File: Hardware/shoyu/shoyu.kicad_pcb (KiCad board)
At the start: 2 copper layers, 58 parts, among them J1 5/9V Connector, J2 24V Connector, J3 SHORI OUT, J4 GAMEN_OUT, J5 MAE OUT, J6 AUDIO IN, U1 TPA3255DDVR, U2 TSR 1-24120

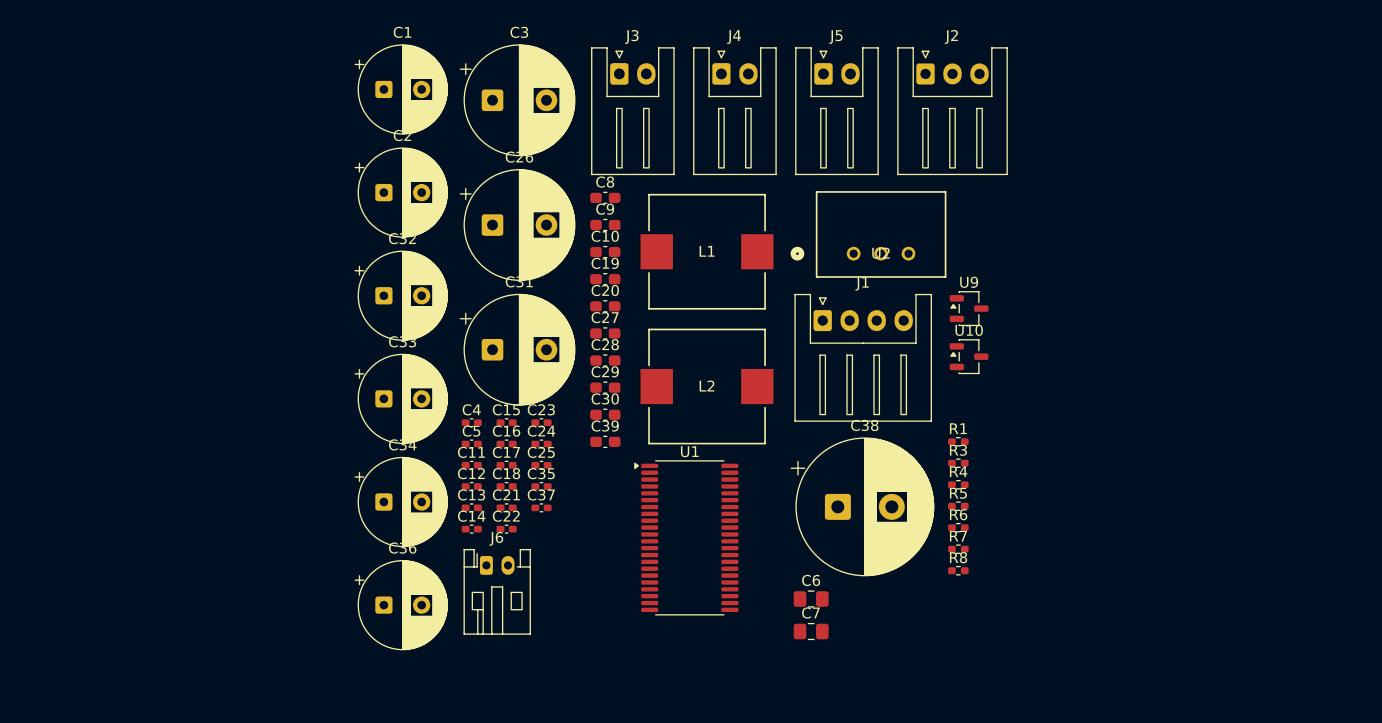
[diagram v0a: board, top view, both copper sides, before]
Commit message: Shoyu: Layout complete
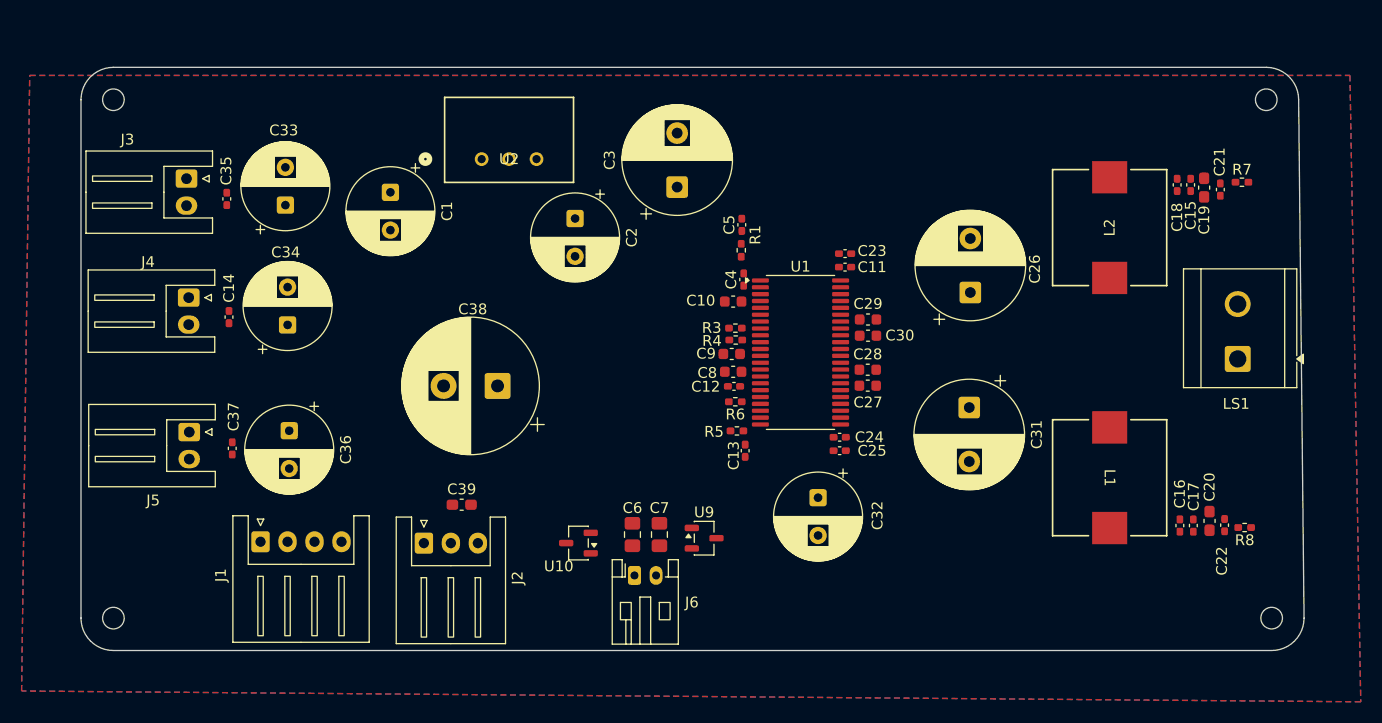
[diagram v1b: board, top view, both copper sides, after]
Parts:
- added H1: MountingHole, MountingHole:MountingHole_2mm, F.Cu at (95.8, 78.0)
- added H2: MountingHole, MountingHole:MountingHole_2mm, F.Cu at (95.8, 126.0)
- added H3: MountingHole, MountingHole:MountingHole_2mm, F.Cu at (202.5, 78.0)
- added H4: MountingHole, MountingHole:MountingHole_2mm, F.Cu at (203.0, 126.0)
- added LS1: Speaker, TerminalBlock_CUI:TerminalBlock_CUI_TB007-508-02_1x02_P5.08mm_Horizontal, F.Cu at (199.9, 102.0)
- C10, C8, C9: footprint Capacitor_SMD:C_0603_1608Metric_Pad1.08x0.95mm_HandSolder -> Capacitor_SMD:C_0603_1608Metric
- C27, C28, C29, C30: value 1uF -> 2.2uF; footprint Capacitor_SMD:C_0603_1608Metric_Pad1.08x0.95mm_HandSolder -> Capacitor_SMD:C_0603_1608Metric
- U2: footprint My Footprints:TSR1-SINGLE_TRP -> My Feet pics:TSR1-SINGLE_TRP
- moved C21 72.4 mm to (198.2, 86.3), turned to -90 degrees
- moved C18 68.1 mm to (194.2, 85.9), turned to 90 degrees
- moved J5 67.4 mm to (102.8, 108.8), turned to -90 degrees
- moved C15 67.1 mm to (195.5, 85.9), turned to 90 degrees
- moved C22 66.5 mm to (198.6, 117.4), turned to -90 degrees
- moved C17 63.8 mm to (195.8, 117.4), turned to 90 degrees
- moved J2 63.6 mm to (124.5, 119.1)
- moved C16 62.8 mm to (194.5, 117.4), turned to 90 degrees
- moved C20 59.4 mm to (197.2, 117.0), turned to 90 degrees
- moved C19 56.1 mm to (196.8, 86.1), turned to 90 degrees
- moved J1 55.9 mm to (109.4, 118.9)
- moved J4 53.5 mm to (102.7, 96.3), turned to -90 degrees
- moved C26 44.7 mm to (175.1, 95.8), turned to 90 degrees
- moved C31 44.5 mm to (175.0, 106.5), turned to -90 degrees
- moved C32 44.3 mm to (161.0, 114.8), turned to -90 degrees
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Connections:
- C6 pad 1: Net-(J6-Pin_2) -> Net-(J6-Pin_1)
- C7 pad 1: Net-(J6-Pin_1) -> Net-(J6-Pin_2)
- J1 pad 2: +5V -> +9V
- J1 pad 4: +9V -> +5V
- U10 pad 1: Net-(J6-Pin_2) -> Net-(J6-Pin_1)
- U9 pad 2: Net-(J6-Pin_1) -> Net-(J6-Pin_2)
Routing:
- added copper zone on B.Cu, net GND
- added copper zone on F.Cu, net GND
- added copper zone on In1.Cu, net GND
- added copper zone on In2.Cu, net GND
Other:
- board outline added: 113.2 x 54 mm
- copper layers 2 -> 4
- board text added: "SHOYU REV 1"
